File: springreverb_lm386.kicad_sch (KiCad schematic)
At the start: 66 parts, among them J1 IN, J10 VR2_3, J11 VR_2_2, J12 To, J13 FromSW, J14 To_Tank, J15 From_Tank, J16 FromGND, J17 From, J18 VR_3_3, J19 VR3_3, J2 INGND, J20 VR4_1, J21 OUT, J22 VR_4_1, J3 GND, J4 Vin, J5 LEDGND, J6 VR1_3, J7 VR_1_1, J8 toC6, J9 toC7, SW1 SW_SPDT, SW2 SW_SPST, U1 TL072, U2 TC1044S, U3 LM386

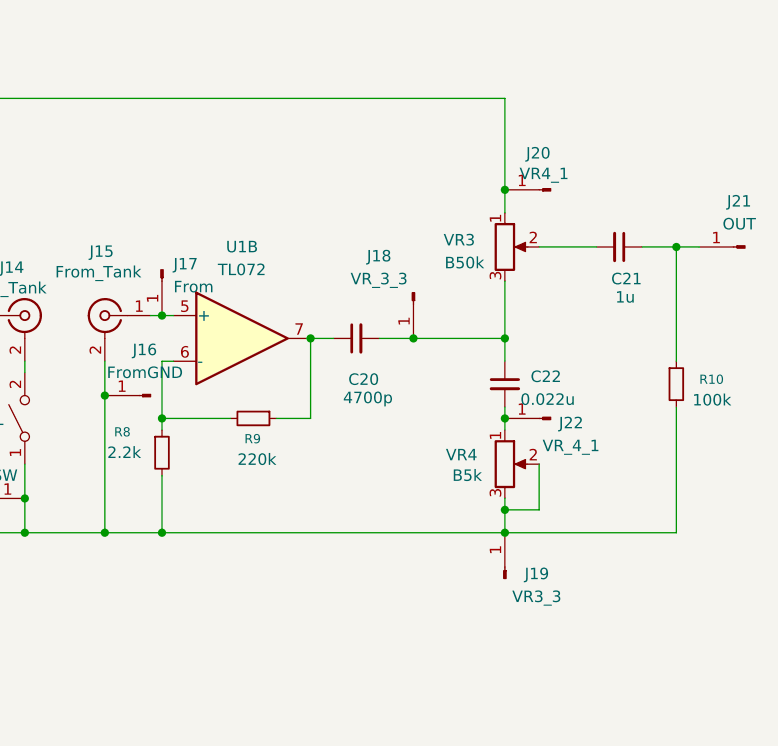
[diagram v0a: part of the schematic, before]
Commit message: トーン回路周りを修正
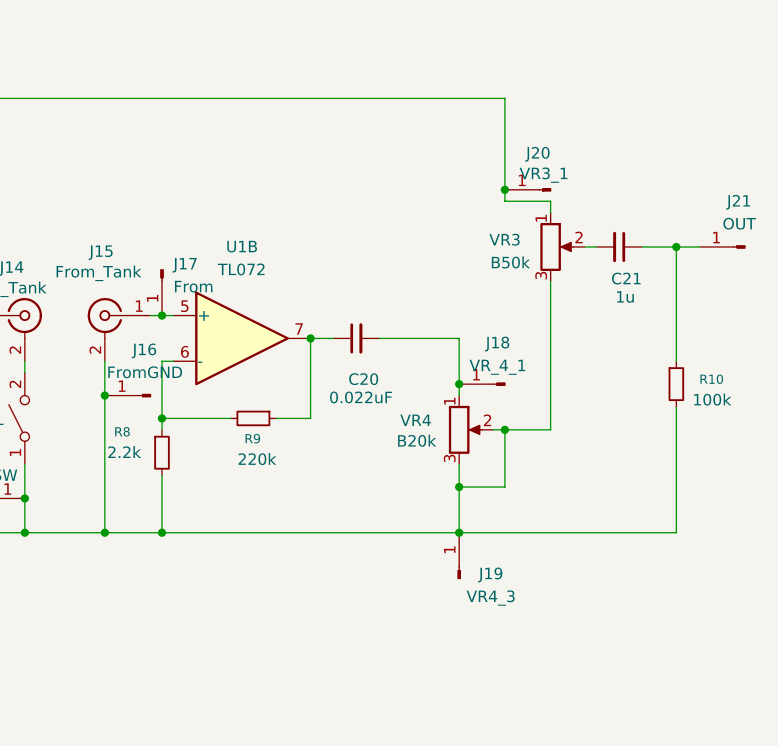
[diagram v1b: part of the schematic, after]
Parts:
- removed C22: 0.022u, MyLibrary:9.3_4.3_p7.5, symbol Device:C_Small
- removed J22: VR_4_1, MyLibrary:PinHeader_1x01_P2.54mm_Vertical, symbol Connector:Conn_01x01_Pin
- C20: value 4700p -> 0.022uF
- J18: value VR_3_3 -> VR_4_1
- J19: value VR3_3 -> VR4_3
- J20: value VR4_1 -> VR3_1
- VR4: value B5k -> B20k
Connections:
- net GND: now also VR3.3
- net at C20.2, J18.1 (Pin_1): now also VR4.1; no longer VR3.3
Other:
- moved on the sheet: J18, J19, VR3, VR4
